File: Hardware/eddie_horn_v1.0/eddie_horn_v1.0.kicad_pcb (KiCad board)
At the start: 2 copper layers, 35 x 36 mm, 20 parts, among them J1 Conn_01x03, J2 Conn_01x02, J3 Conn_01x02, J4 Conn_01x02, Q1 IRF6646

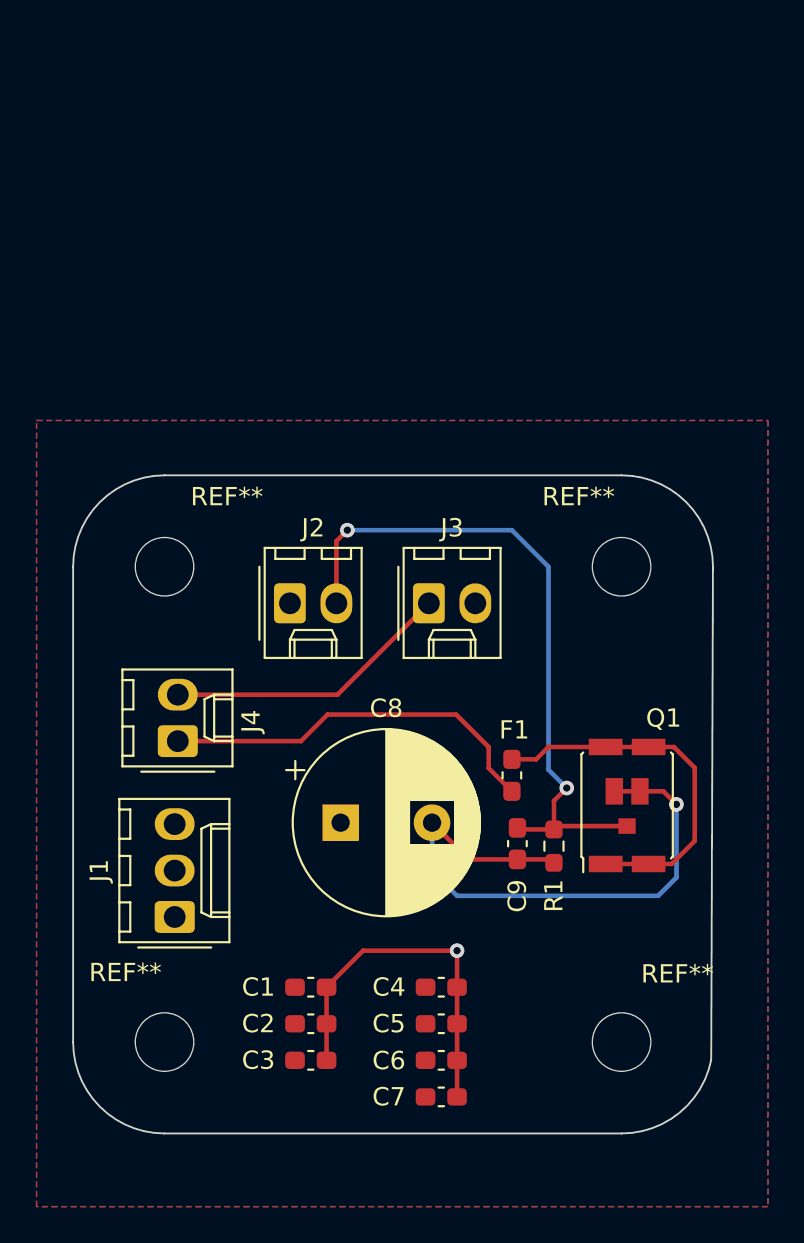
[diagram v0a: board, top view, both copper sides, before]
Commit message: implemented changes to board and code
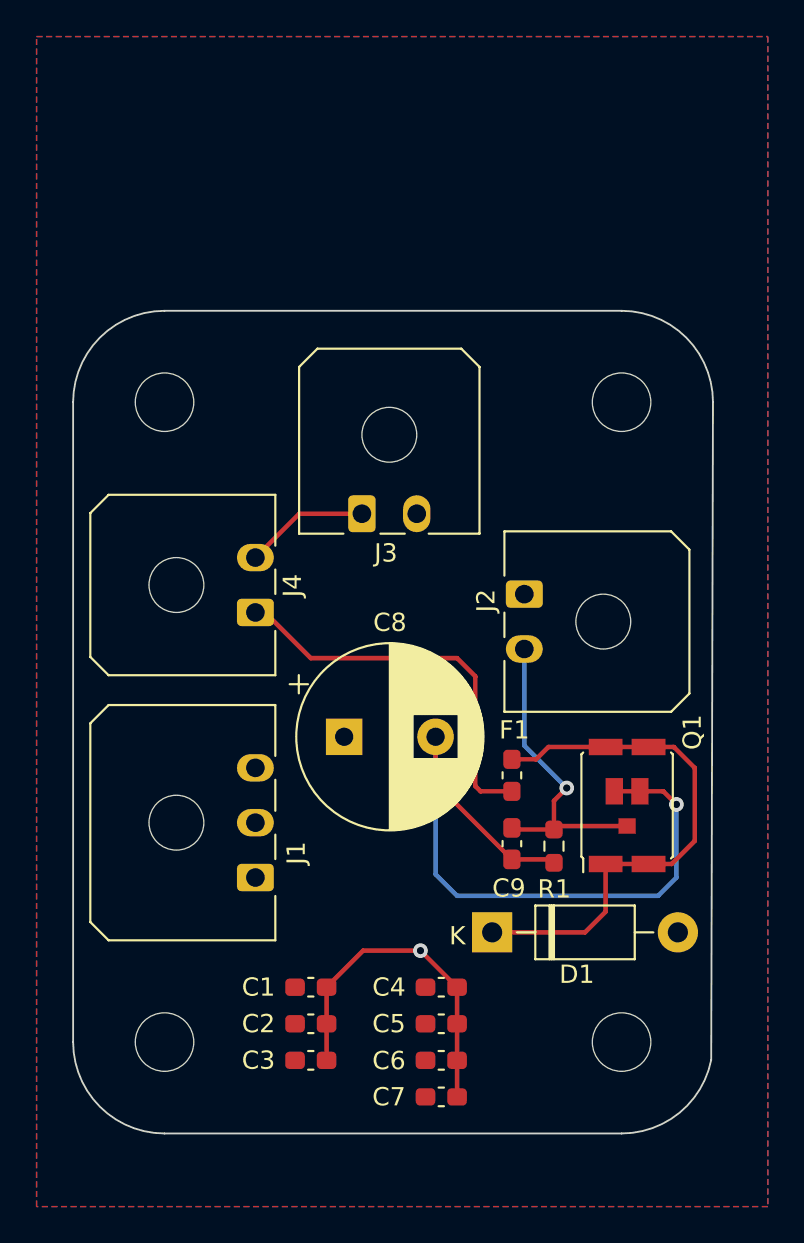
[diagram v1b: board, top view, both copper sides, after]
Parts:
- added D1: 1N4002, Diode_THT:D_DO-41_SOD81_P10.16mm_Horizontal, F.Cu at (145.9, 90.0)
- J1: footprint Connector_Molex:Molex_KK-254_AE-6410-03A_1x03_P2.54mm_Vertical -> Connector_Molex:Molex_Micro-Fit_3.0_43650-0300_1x03_P3.00mm_Horizontal
- J2, J3, J4: footprint Connector_Molex:Molex_KK-254_AE-6410-02A_1x02_P2.54mm_Vertical -> Connector_Molex:Molex_Micro-Fit_3.0_43650-0200_1x02_P3.00mm_Horizontal
- moved J2 12.8 mm to (147.7, 71.5), turned to -90 degrees
- moved REF** 9.00 mm to (153.0, 61.0)
- moved REF** 9.00 mm to (128.0, 61.0)
- moved J4 8.22 mm to (133.0, 72.5)
- moved J3 6.12 mm to (138.8, 67.1)
- moved J1 4.91 mm to (133.0, 87.0)
- moved C8 4.70 mm to (137.8, 79.3)
- moved C9 0.30 mm to (147.0, 85.1)
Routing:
- net HRN_CTRL: track 37.3 -> 17.2 mm, vias 2 -> 1
- net Net-(D1-K): track 20.2 -> 29.4 mm
- net Net-(J3-Pin_1): track 15.8 -> 6.82 mm
- net GND: track 52.2 -> 58.9 mm
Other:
- board size 35 x 36 mm -> 35 x 45 mm
